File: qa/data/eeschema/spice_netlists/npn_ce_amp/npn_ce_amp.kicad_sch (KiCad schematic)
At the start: 10 parts, among them Q1 QNPN

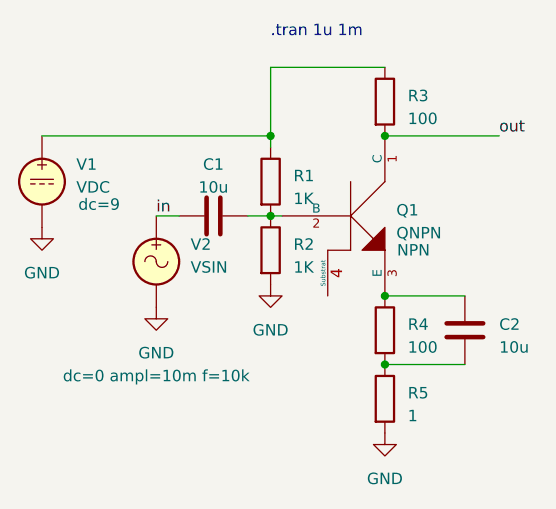
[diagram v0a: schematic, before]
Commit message: Sim: Remove inference from Reference and Value
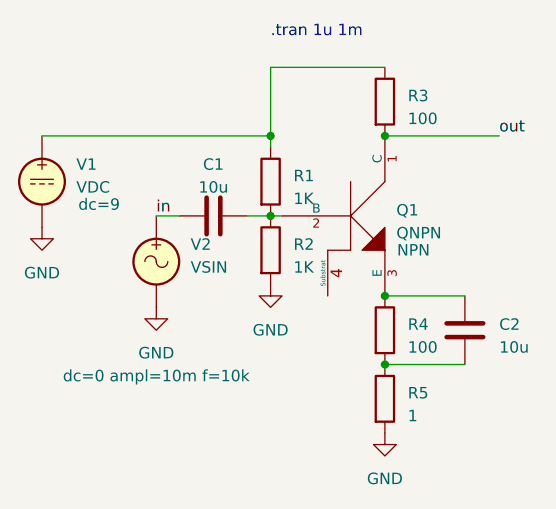
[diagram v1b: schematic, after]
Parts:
- C1, C2: Sim_Device (none) -> C
- R1, R2, R3, R4, R5: Sim_Device (none) -> R
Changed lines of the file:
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@@
+      (effects (font (size 1.27 1.27)) hide)
+    )
+    (property "Sim_Device" "C" (at 120.65 88.9 90)
       (effects (font (size 1.27 1.27)) hide)
     )
@@
       (effects (font (size 1.27 1.27)) hide)
     )
+    (property "Sim_Device" "C" (at 148.59 101.6 0)
+      (effects (font (size 1.27 1.27)) hide)
+    )
     (pin "1")
     (pin "2")
@@
     )
     (property "Datasheet" "~" (at 139.7 76.2 0)
+      (effects (font (size 1.27 1.27)) hide)
+    )
+    (property "Sim_Device" "R" (at 139.7 76.2 0)
       (effects (font (size 1.27 1.27)) hide)
     )
@@
       (effects (font (size 1.27 1.27)) hide)
     )
+    (property "Sim_Device" "R" (at 139.7 101.6 0)
+      (effects (font (size 1.27 1.27)) hide)
+    )
     (pin "1")
     (pin "2")
@@
       (effects (font (size 1.27 1.27)) hide)
     )
+    (property "Sim_Device" "R" (at 127 85.09 0)
+      (effects (font (size 1.27 1.27)) hide)
+    )
     (pin "1")
     (pin "2")
@@
       (effects (font (size 1.27 1.27)) hide)
     )
+    (property "Sim_Device" "R" (at 139.7 109.22 0)
+      (effects (font (size 1.27 1.27)) hide)
+    )
     (pin "1")
     (pin "2")
@@
       (effects (font (size 1.27 1.27)) hide)
     )
+    (property "Sim_Device" "R" (at 127 92.71 0)
+      (effects (font (size 1.27 1.27)) hide)
+    )
